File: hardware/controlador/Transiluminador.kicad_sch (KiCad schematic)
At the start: 89 parts, among them J10 USB_B_Micro, J7 HDR-3x1, J9 HDR-3x1, Q1 Q_PMOS_GSD, Q4 Q_Dual_NPN_NPN_BRT_E1B1C2E2B2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, SW2 SW_DIP_x02, SW3 SW_DIP_x02, SW4 SW_DIP_x02, SW5 SW_DIP_x02, U10 ESP32-WROOM-32D, U4 MT3608, U6 AP2112K-3.3, U7 AP2112K-3.3, U8 AP2112K-3.3, U9 CH340C

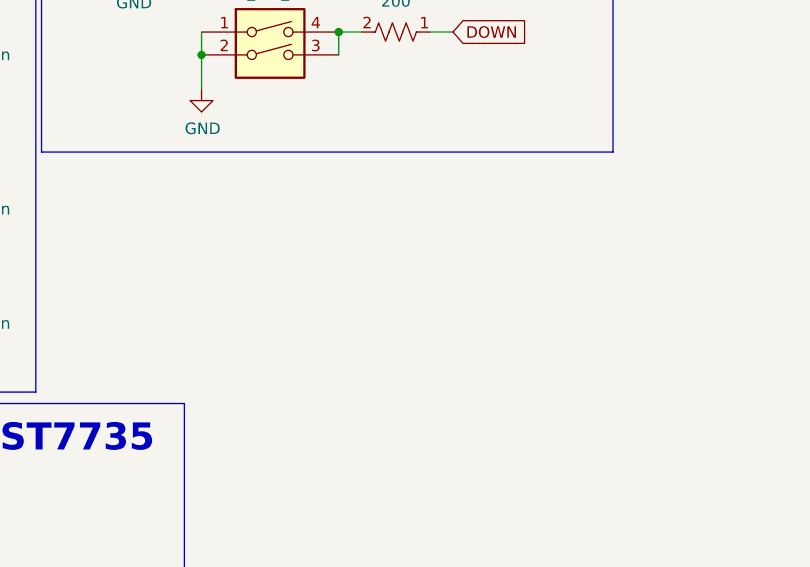
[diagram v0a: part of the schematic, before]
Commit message: sensorluz
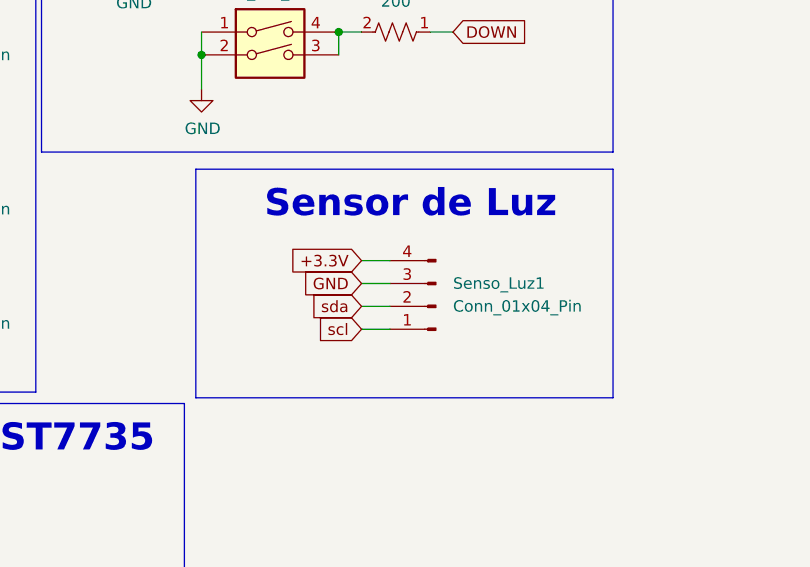
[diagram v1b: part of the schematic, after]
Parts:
- added Senso_Luz1: Conn_01x04_Pin, Connector_JST:JST_XH_B4B-XH-A_1x04_P2.50mm_Vertical, symbol Connector:Conn_01x04_Pin
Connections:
- net +3V3: now also Senso_Luz1.4 (Pin_4)
- net GND: now also Senso_Luz1.3 (Pin_3)
- net scl: now also Senso_Luz1.1 (Pin_1)
- net sda: now also Senso_Luz1.2 (Pin_2)
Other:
- note added: "Sensor de Luz"
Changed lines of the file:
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@@
     (stroke (width 0) (type default))
   )
+  (wire (pts (xy 485.14 80.645) (xy 488.315 80.645))
+    (stroke (width 0) (type default))
+  )
   (wire (pts (xy 187.325 109.855) (xy 189.865 109.855))
     (stroke (width 0) (type default))
@@
     (stroke (width 0) (type default))
   )
+  (wire (pts (xy 485.14 73.025) (xy 488.315 73.025))
+    (stroke (width 0) (type default))
+  )
   (wire (pts (xy 478.79 33.655) (xy 474.98 33.655))
     (stroke (width 0) (type default))
@@
     (stroke (width 0) (type default))
   )
+  (wire (pts (xy 485.14 75.565) (xy 488.315 75.565))
+    (stroke (width 0) (type default))
+  )
   (wire (pts (xy 156.845 121.92) (xy 156.845 120.65))
     (stroke (width 0) (type default))
@@
     (stroke (width 0) (type default))
   )
+  (wire (pts (xy 485.14 78.105) (xy 488.315 78.105))
+    (stroke (width 0) (type default))
+  )
   (wire (pts (xy 212.725 123.825) (xy 212.725 122.555))
     (stroke (width 0) (type default))
@@
     (fill (type none))
   )
+  (rectangle (start 466.725 62.865) (end 513.08 88.265)
+    (stroke (width 0) (type default))
+    (fill (type none))
+  )
   (rectangle (start 129.54 90.17) (end 240.03 160.02)
     (stroke (width 0) (type default))
@@
     (effects (font (size 2.9972 2.9972) (thickness 0.5994) bold) (justify left bottom))
   )
+  (text "Sensor de Luz" (at 474.345 68.58 0)
+    (effects (font (size 2.9972 2.9972) (thickness 0.5994) bold) (justify left bottom))
+  )
   (text "TRANSILLUMINATOR CONTROLLER" (at 801.37 201.295 0)
     (effects (font (size 2.0066 2.0066)) (justify left bottom))
@@
     )
   )
+  (global_label "+3.3V" (shape input) (at 485.14 73.025 180) (fields_autoplaced)
+    (effects (font (size 1.27 1.27)) (justify right))
+    (property "Intersheetrefs" "${INTERSHEET_REFS}" (at 476.47 73.025 0)
+      (effects (font (size 1.27 1.27)) (justify right) hide)
+    )
+  )
   (global_label "+5V" (shape input) (at 93.98 135.89 0) (fields_autoplaced)
     (effects (font (size 1.27 1.27)) (justify left))
@@
     )
   )
+  (global_label "GND" (shape input) (at 485.14 75.565 180) (fields_autoplaced)
+    (effects (font (size 1.27 1.27)) (justify right))
+    (property "Intersheetrefs" "${INTERSHEET_REFS}" (at 478.2843 75.565 0)
+      (effects (font (size 1.27 1.27)) (justify right) hide)
+    )
+  )
   (global_label "V_DD" (shape input) (at 419.735 46.355 180) (fields_autoplaced)
     (effects (font (size 1.27 1.27)) (justify right))
@@
     )
   )
+  (global_label "scl" (shape input) (at 485.14 80.645 180) (fields_autoplaced)
+    (effects (font (size 1.27 1.27)) (justify right))
+    (property "Intersheetrefs" "${INTERSHEET_REFS}" (at 479.3729 80.645 0)
+      (effects (font (size 1.27 1.27)) (justify right) hide)
+    )
+  )
   (global_label "V_in" (shape input) (at 26.035 50.8 180) (fields_autoplaced)
     (effects (font (size 1.27 1.27)) (justify right))
@@
     )
   )
+  (global_label "sda" (shape input) (at 485.14 78.105 180) (fields_autoplaced)
+    (effects (font (size 1.27 1.27)) (justify right))
+    (property "Intersheetrefs" "${INTERSHEET_REFS}" (at 478.8287 78.105 0)
+      (effects (font (size 1.27 1.27)) (justify right) hide)
+    )
+  )
   (global_label "RES" (shape input) (at 427.355 119.38 0) (fields_autoplaced)
     (effects (font (size 1.27 1.27)) (justify left))
@@
         )
       )
+    )
+  )
+  (symbol (lib_id "Connector:Conn_01x04_Pin") (at 493.395 78.105 180) (unit 1)
+    (in_bom yes) (on_board yes) (dnp no) (fields_autoplaced)
+    (property "Reference" "Senso_Luz1" (at 495.3 75.565 0)
+      (effects (font (size 1.27 1.27)) (justify right))
+    )
+    (property "Value" "Conn_01x04_Pin" (at 495.3 78.105 0)
+      (effects (font (size 1.27 1.27)) (justify right))
+    )
+    (property "Footprint" "Connector_JST:JST_XH_B4B-XH-A_1x04_P2.50mm_Vertical" (at 493.395 78.105 0)
+      (effects (font (size 1.27 1.27)) hide)
+    )
+    (property "Datasheet" "~" (at 493.395 78.105 0)
+      (effects (font (size 1.27 1.27)) hide)
+    )
+    (pin "1")
+    (pin "4")
+    (pin "2")
+    (pin "3")
+    (instances
+      (project "Transiluminador"
+        (path "/3bccb558-cfc1-47b0-87de-a688fdd981c6"
+          (reference "Senso_Luz1") (unit 1)
+        )
+      )
